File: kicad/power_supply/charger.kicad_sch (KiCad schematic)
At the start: 17 parts

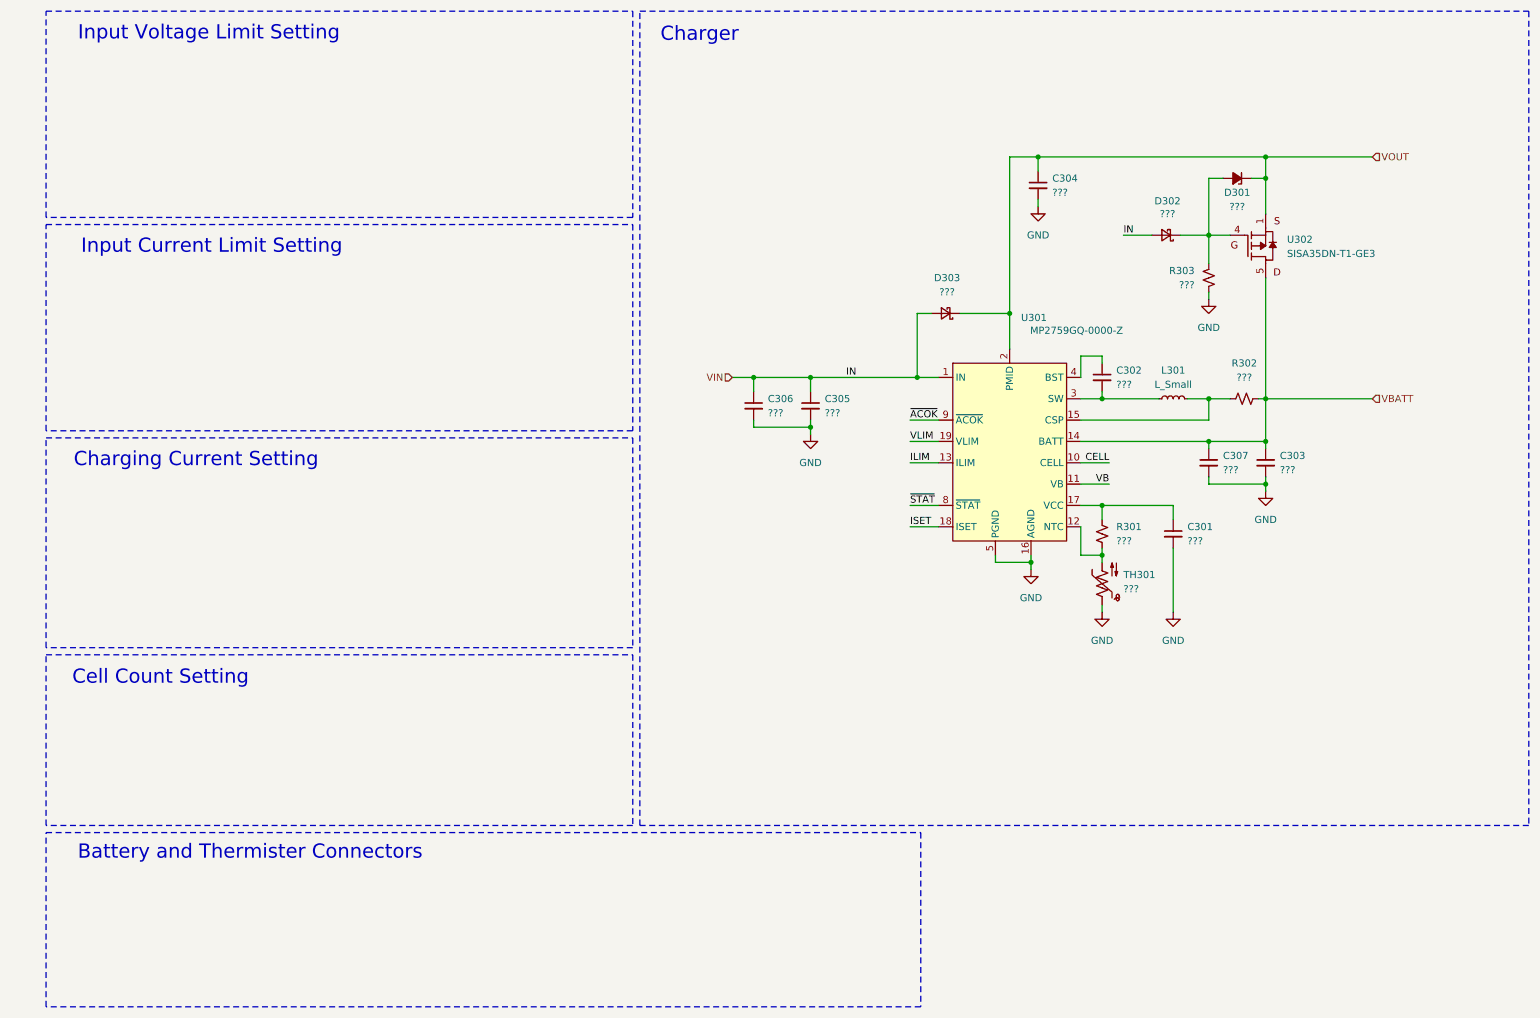
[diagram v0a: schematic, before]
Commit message: schematic capture
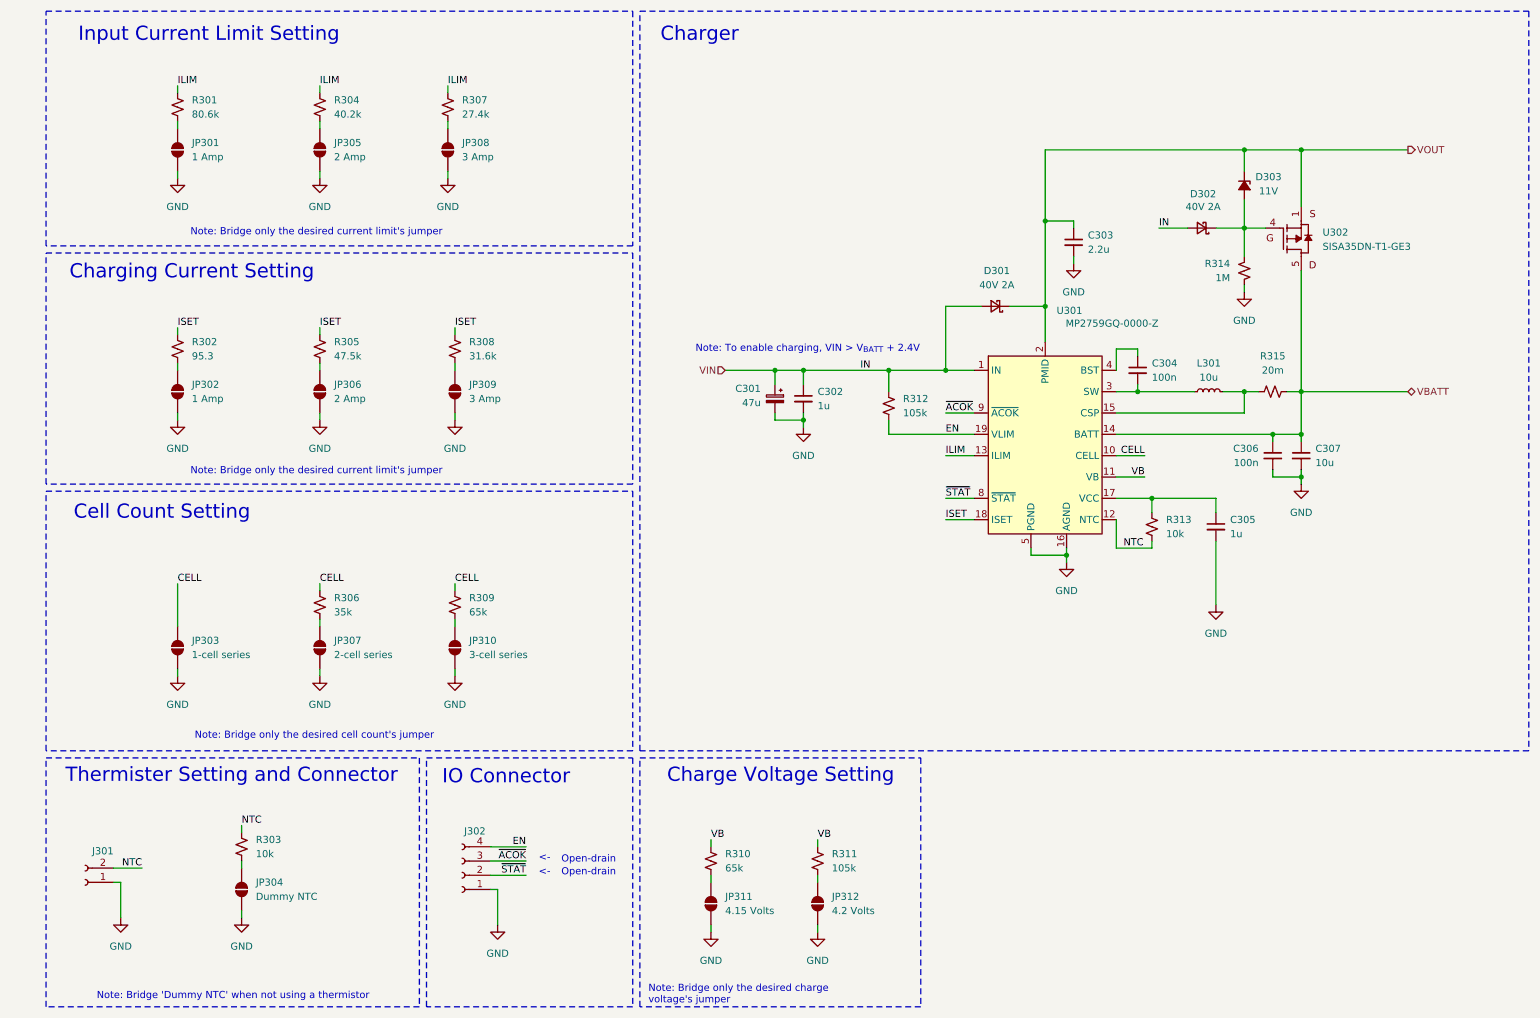
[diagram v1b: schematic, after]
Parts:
- removed C306: ???, symbol Device:C_Small
- removed TH301: ???, symbol Device:Thermistor_NTC_US
- added C301: 47u, symbol Device:C_Polarized_Small
- added J301: Conn_01x02_Socket, symbol Connector:Conn_01x02_Socket
- added J302: Conn_01x04_Socket, symbol Connector:Conn_01x04_Socket
- added JP301, JP302: 1 Amp, symbol Jumper:SolderJumper_2_Open
- added JP303: 1-cell series, symbol Jumper:SolderJumper_2_Open
- added JP304: Dummy NTC, symbol Jumper:SolderJumper_2_Open
- added JP305, JP306: 2 Amp, symbol Jumper:SolderJumper_2_Open
- added JP307: 2-cell series, symbol Jumper:SolderJumper_2_Open
- added JP308, JP309: 3 Amp, symbol Jumper:SolderJumper_2_Open
- added JP310: 3-cell series, symbol Jumper:SolderJumper_2_Open
- added JP311: 4.15 Volts, symbol Jumper:SolderJumper_2_Open
- added JP312: 4.2 Volts, symbol Jumper:SolderJumper_2_Open
- added R301: 80.6k, symbol Device:R_Small_US
- added R302: 95.3, symbol Device:R_Small_US
- added R303: 10k, symbol Device:R_Small_US
- added R304: 40.2k, symbol Device:R_Small_US
- added R305: 47.5k, symbol Device:R_Small_US
- added R306: 35k, symbol Device:R_Small_US
- added R307: 27.4k, symbol Device:R_Small_US
- added R308: 31.6k, symbol Device:R_Small_US
- added R309, R310: 65k, symbol Device:R_Small_US
- added R311, R312: 105k, symbol Device:R_Small_US
- C302: renamed from C305; value ??? -> 1u
- C303: renamed from C304; value ??? -> 2.2u
- C304: renamed from C302; value ??? -> 100n
- C305: renamed from C301; value ??? -> 1u
- C306: renamed from C307; value ??? -> 100n
- C307: renamed from C303; value ??? -> 10u
- D301: renamed from D303; value ??? -> 40V 2A
- D302: value ??? -> 40V 2A
- D303: renamed from D301; value ??? -> 11V
- L301: value L_Small -> 10u
- R313: renamed from R301; value ??? -> 10k
- R314: renamed from R303; value ??? -> 1M
- R315: renamed from R302; value ??? -> 20m
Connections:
- net CELL: now also JP303.2 (B), R306.1, R309.1
- net GND: now also C301.2, J301.1 (Pin_1), J302.1 (Pin_1), JP301.1 (A), JP302.1 (A), JP303.1 (A), JP304.1 (A), JP305.1 (A), JP306.1 (A), JP307.1 (A), JP308.1 (A), JP309.1 (A), JP310.1 (A), JP311.1 (A), JP312.1 (A)
- net ILIM: now also R301.1, R304.1, R307.1
- net ISET: now also R302.1, R305.1, R308.1
- net VB: now also R310.1, R311.1
- net VIN: now also C301.1, R312.1
- net ~{ACOK}: now also J302.3 (Pin_3)
- net ~{STAT}: now also J302.2 (Pin_2)
- net NTC: now reaches R313.2, U301.12 (NTC)
- net NTC: now also J301.2 (Pin_2), R303.1
- net VLIM renamed EN
- net EN: now also J302.4 (Pin_4), R312.2
- new net: JP309.2 (B), R308.2
- new net: JP312.2 (B), R311.2
- new net: JP301.2 (B), R301.2
- new net: JP308.2 (B), R307.2
- new net: JP306.2 (B), R305.2
- new net: JP311.2 (B), R310.2
- new net: JP310.2 (B), R309.2
- new net: JP307.2 (B), R306.2
- new net: JP304.2 (B), R303.2
- new net: JP302.2 (B), R302.2
- new net: JP305.2 (B), R304.2
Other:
- note added: "<-"
- note added: "Charge Voltage Setting"
- note added: "IO Connector"
- note added: "Note: Bridge 'Dummy NTC' when not using a thermistor"
- note added: "Note: Bridge only the desired cell count's jumper"
- note added: "Note: Bridge only the desired charge voltage's jumper"
- note added: "Note: Bridge only the desired current limit's jumper"
- note added: "Note: To enable charging, VIN > V_{BATT} + 2.4V"
- note added: "Open-drain"
- note added: "Thermister Setting and Connector"
- note removed: "Battery and Thermister Connectors"
- note removed: "Input Voltage Limit Setting"
- moved on the sheet: C302, C303, C304, C305, C306, C307, D301, D302, D303, L301, R313, R314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
